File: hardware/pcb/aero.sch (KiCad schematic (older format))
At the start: 9 parts

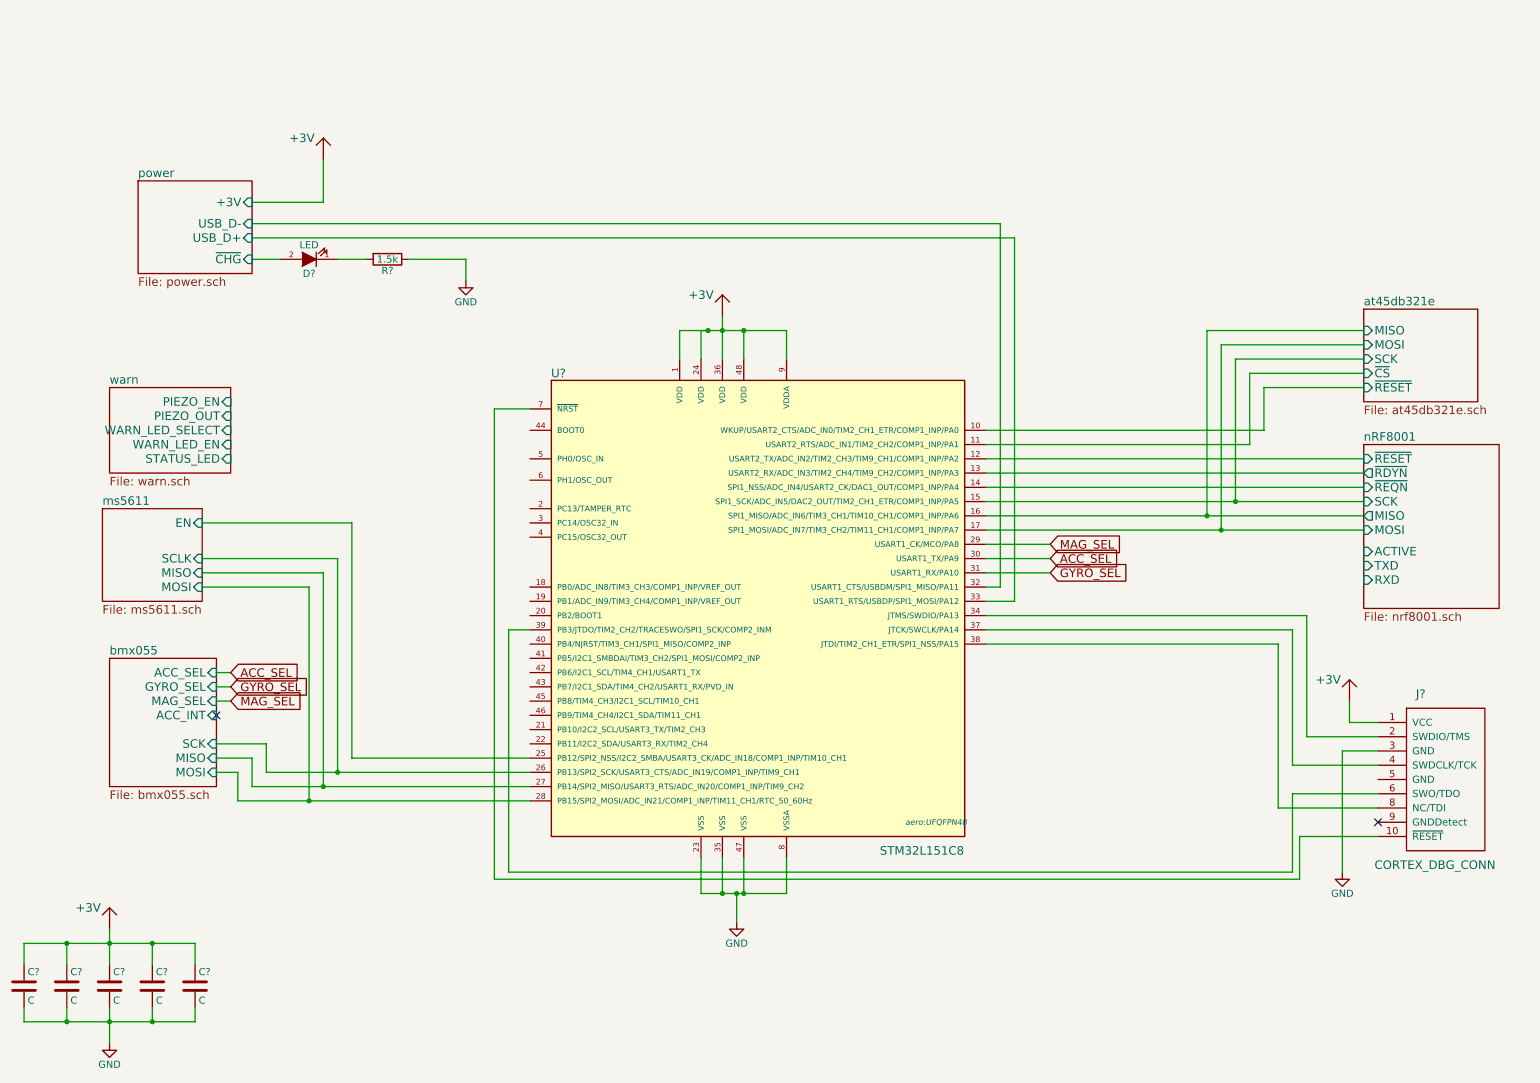
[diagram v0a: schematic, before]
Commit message: schematic updates
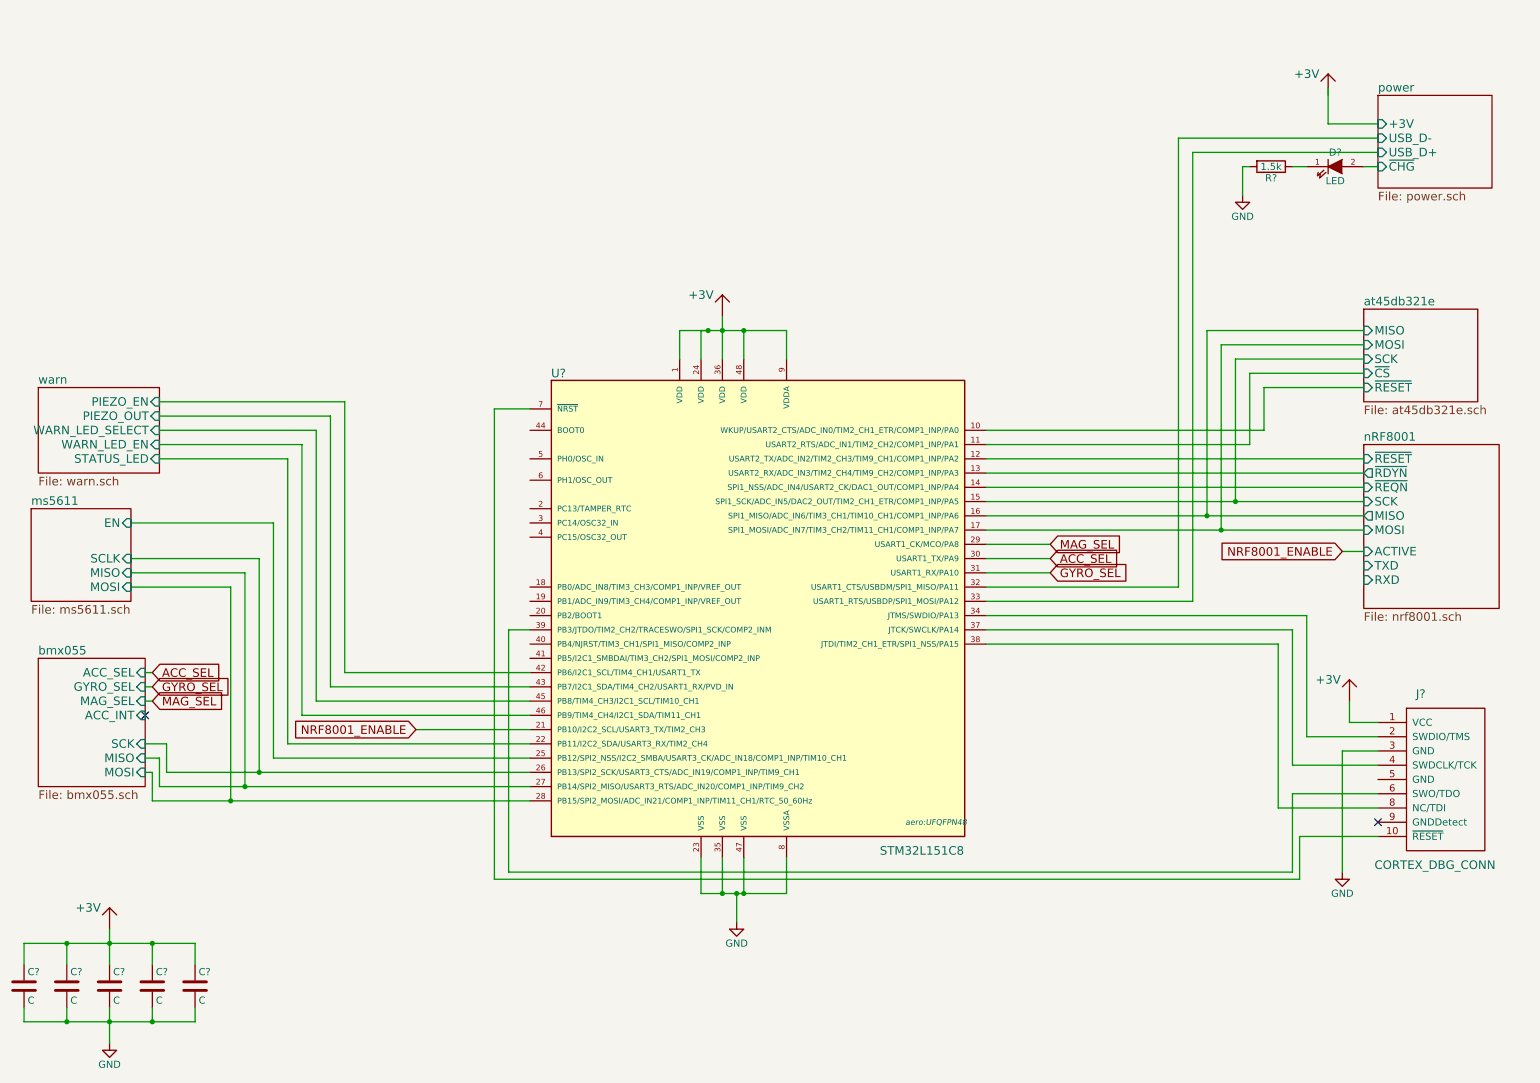
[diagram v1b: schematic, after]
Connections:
- net GND: now also R?.2; no longer R?.1
- net warn/PIEZO_EN: now also U?.42 (PB6/I2C1_SCL/TIM4_CH1/USART1_TX)
- net warn/PIEZO_OUT: now also U?.43 (PB7/I2C1_SDA/TIM4_CH2/USART1_RX/PVD_IN)
- net warn/STATUS_LED: now also U?.22 (PB11/I2C2_SDA/USART3_RX/TIM2_CH4)
- net warn/WARN_LED_EN: now also U?.46 (PB9/TIM4_CH4/I2C1_SDA/TIM11_CH1)
- net warn/WARN_LED_SELECT: now also U?.45 (PB8/TIM4_CH3/I2C1_SCL/TIM10_CH1)
- net NRF8001_ENABLE: now reaches U?.21 (PB10/I2C2_SCL/USART3_TX/TIM2_CH3)
- net at D?.1 (K): now also R?.1; no longer R?.2
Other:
- moved on the sheet: D?, R?

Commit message: schematic updates
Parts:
- added 10k, R? (x2): R, symbol R
- added C? (x4): C, symbol C
- added Y? (x2): Crystal_Small, symbol Crystal_Small
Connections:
- net labels added: SWO, ~NRST
- wire segments 119 -> 167
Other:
- moved on the sheet: D?, J?, R?
